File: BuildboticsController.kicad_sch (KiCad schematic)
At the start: 0 parts

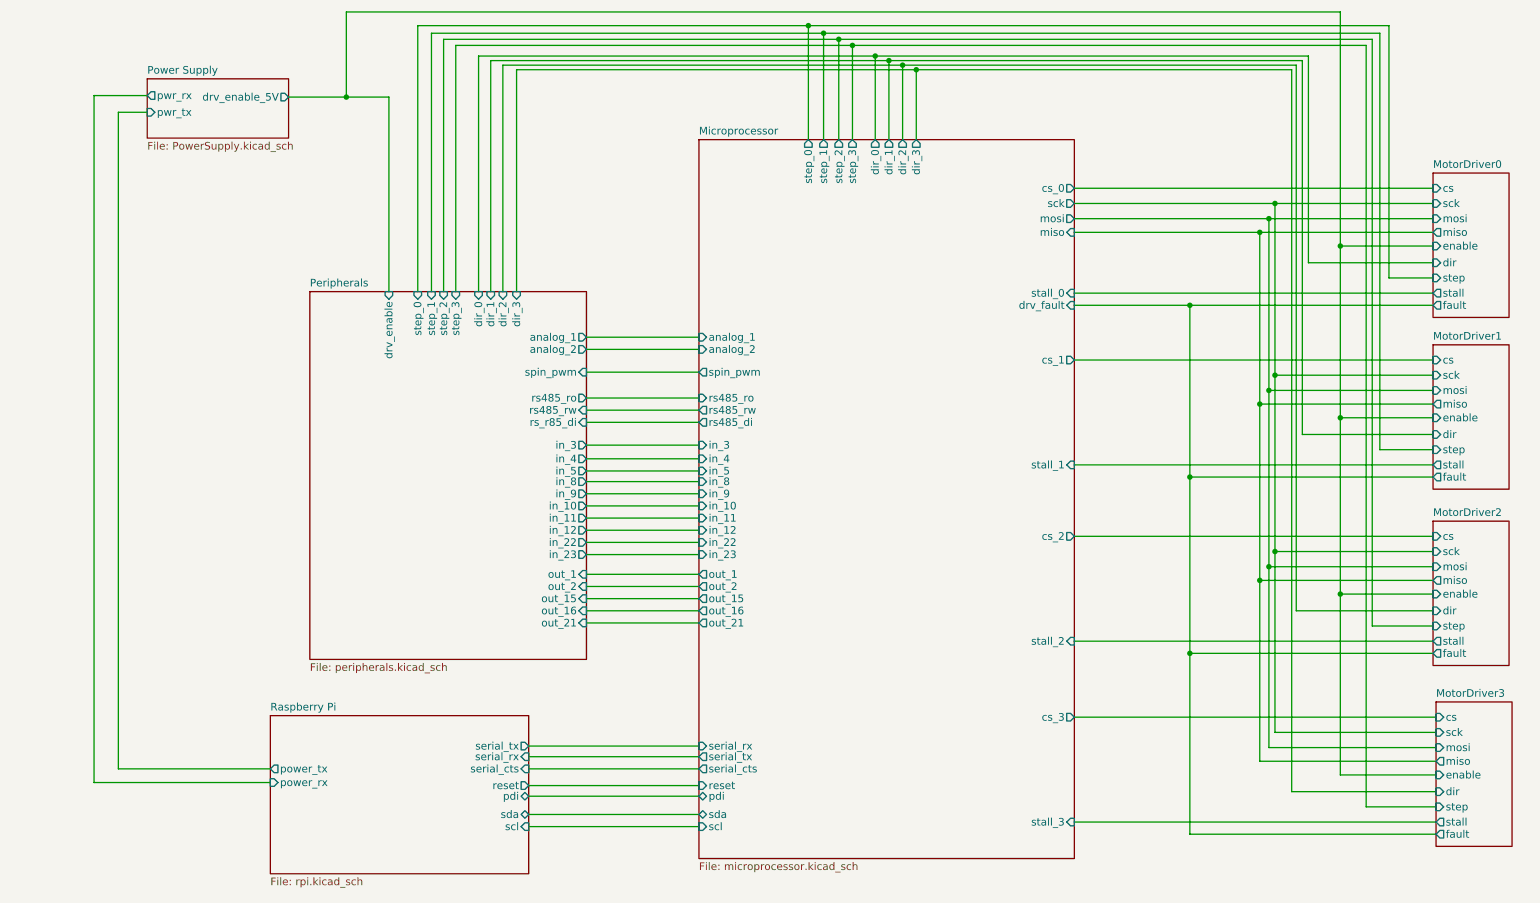
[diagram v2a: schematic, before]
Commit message: corrections after first KiCad build
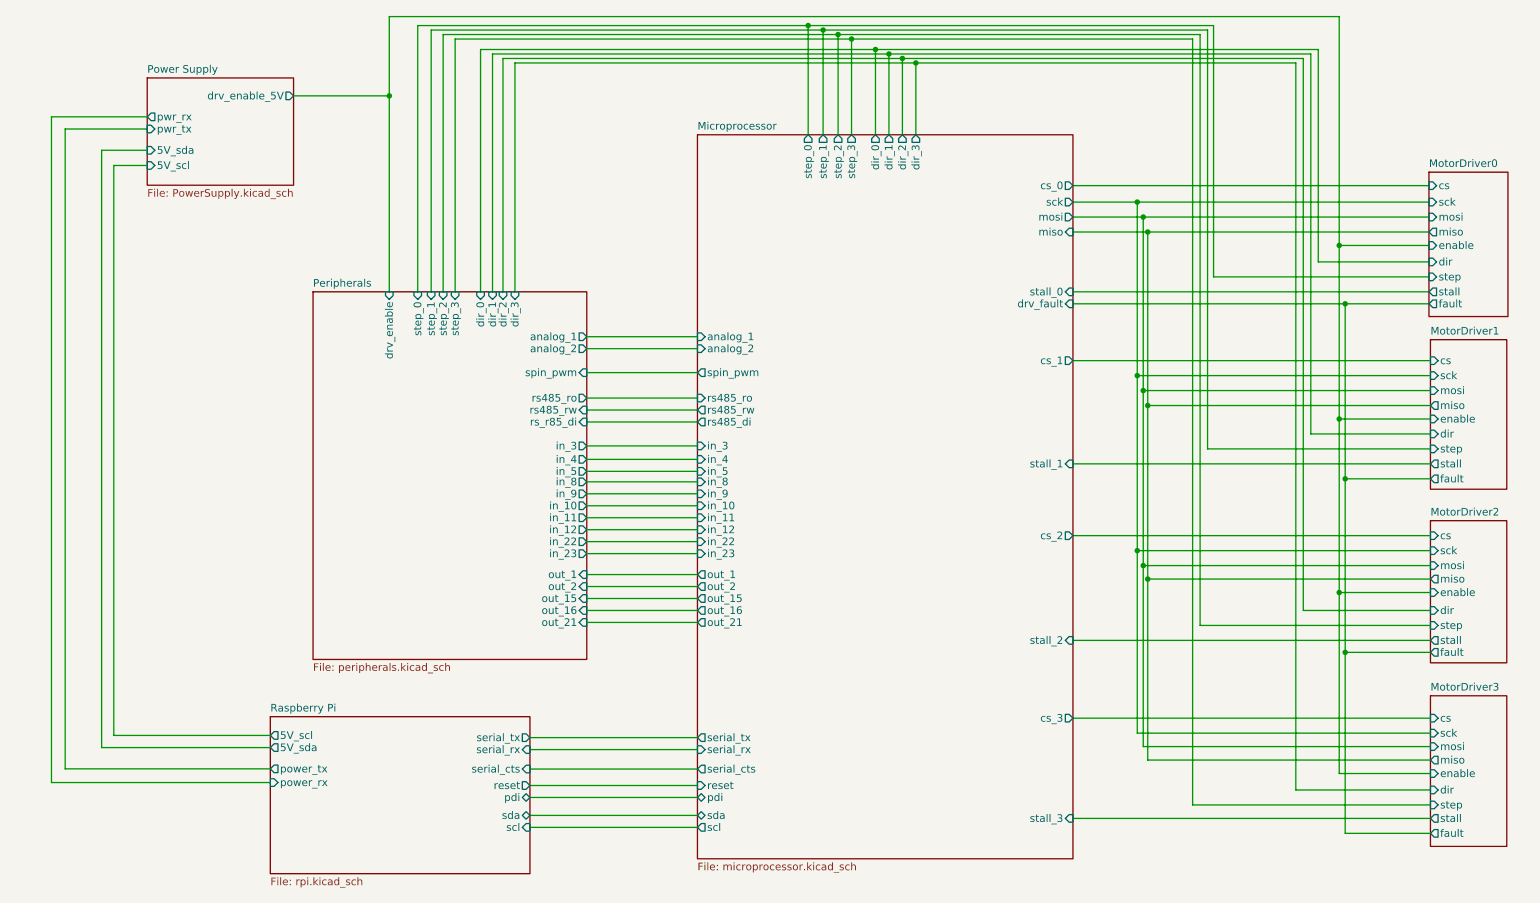
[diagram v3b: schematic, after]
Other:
- sheet Power Supply ports: added 5V_scl, 5V_sda; removed none
- sheet Raspberry Pi ports: added 5V_scl, 5V_sda; removed none

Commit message: put all schematics on 50 mil grid
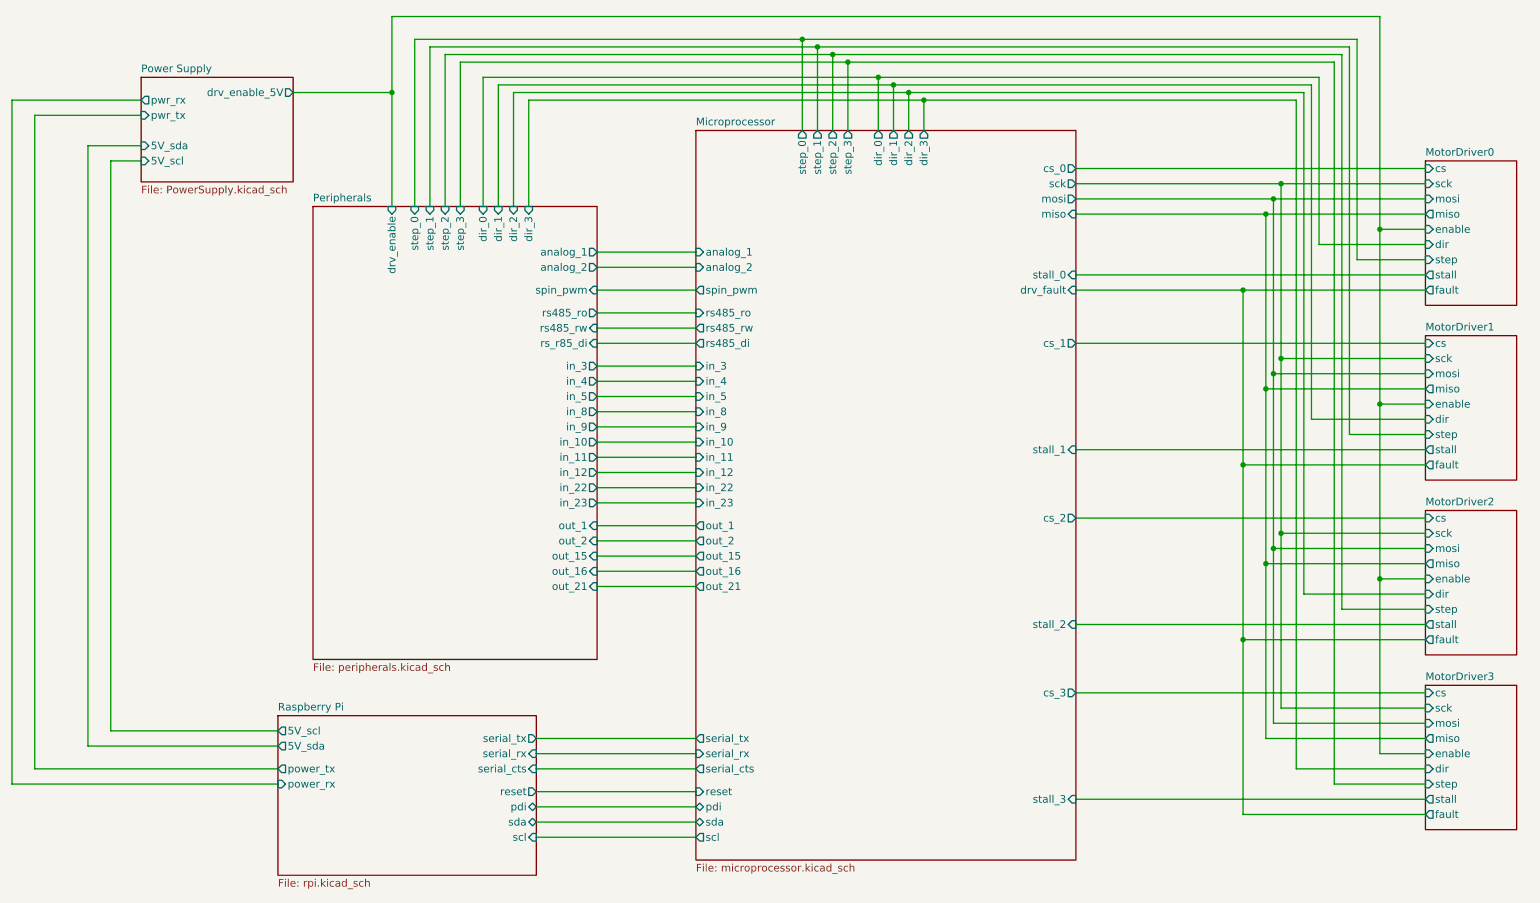
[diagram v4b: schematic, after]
